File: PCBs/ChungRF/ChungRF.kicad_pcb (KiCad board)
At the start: 4 copper layers, 28.4 x 52.3 mm, 9 parts, among them J1 JST-SM04B-SRSS, J2 Conn_Coaxial, U1 KB2040, U2 E22-900M30S

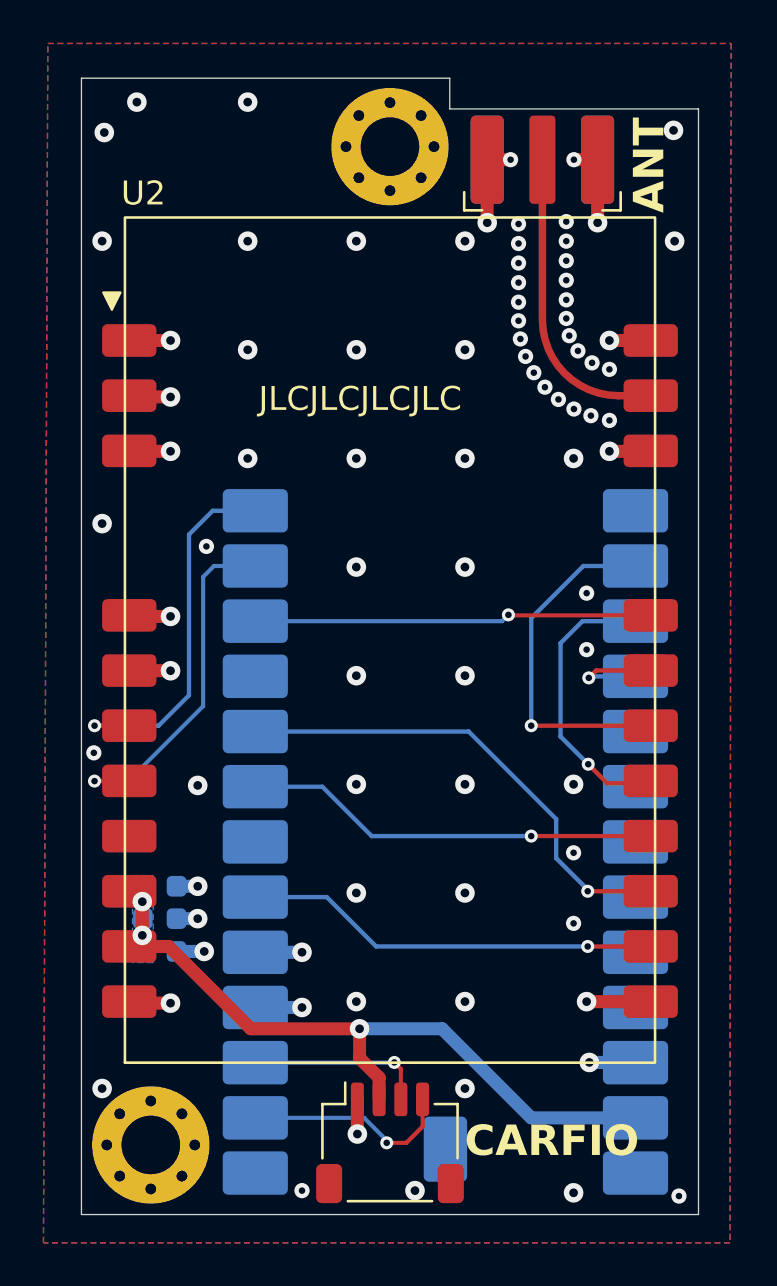
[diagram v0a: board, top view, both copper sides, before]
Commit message: ChungRF R3
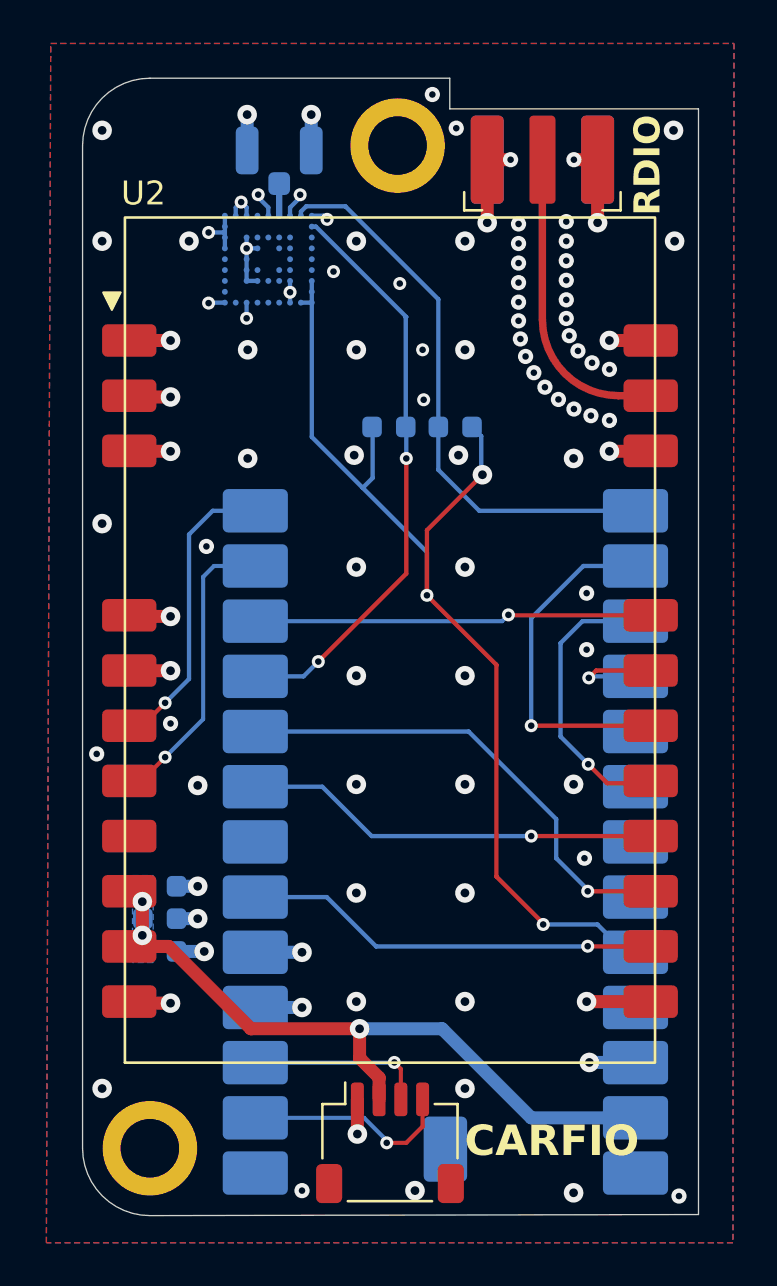
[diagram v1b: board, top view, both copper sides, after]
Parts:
- added J3: uFL, Connector_Coaxial:U.FL_Hirose_U.FL-R-SMT-1_Vertical, B.Cu at (160.4, 65.3)
- added R1: 5.1k, Capacitor_SMD:C_0603_1608Metric, B.Cu at (165.5, 77.5)
- added R2: 5.1k, Capacitor_SMD:C_0603_1608Metric, B.Cu at (168.6, 77.5)
- added U3: ZOE-M8Q, RF_GPS:ublox_ZOE_M8, B.Cu at (159.9, 69.8)
- H1, H2: value 2.7mm_M2.5_Pad_Via -> 2.7mm_M2.5_Pad; footprint MountingHole:MountingHole_2.7mm_M2.5_Pad_Via -> besser_footprints:M2.5_2.7mm_hole
- moved H1 0.35 mm to (165.9, 64.6)
- moved H2 0.16 mm to (154.5, 110.8)
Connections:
- U1 pad 10: unconnected-(U1-D6-Pad10) -> /GNSS_SCL
- U1 pad 14: unconnected-(U1-D10-Pad14) -> /GNSS_SDA
- U1 pad 22: unconnected-(U1-3v3-Pad22) -> +3V3
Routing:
- net +3V3: track 0.00 -> 51.3 mm, vias 0 -> 3
- net /GNSS_SCL: track 0.00 -> 26.8 mm, vias 0 -> 2
- net /GNSS_SDA: track 0.00 -> 26.1 mm
- net GND: track 37.4 -> 53.2 mm, vias 85 -> 100
- net /RXEN: track 17.4 -> 13.8 mm
- net /TXEN: track 16.6 -> 13.7 mm
- net /RF_GNSS: track 0.00 -> 1.48 mm
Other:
- board size 28.4 x 52.3 mm -> 28.3 x 52.3 mm
- board text added: "GNSS"
- board text added: "R3 11-2024"
- board text added: "RDIO"
- board text removed: "ANT"
- board text removed: "JLCJLCJLCJLC"
- board text removed: "R3 10-2024"
